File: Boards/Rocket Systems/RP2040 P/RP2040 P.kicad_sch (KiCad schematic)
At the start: 2 parts, among them J1 Conn_01x20_Pin, J3 Conn_01x18_Pin

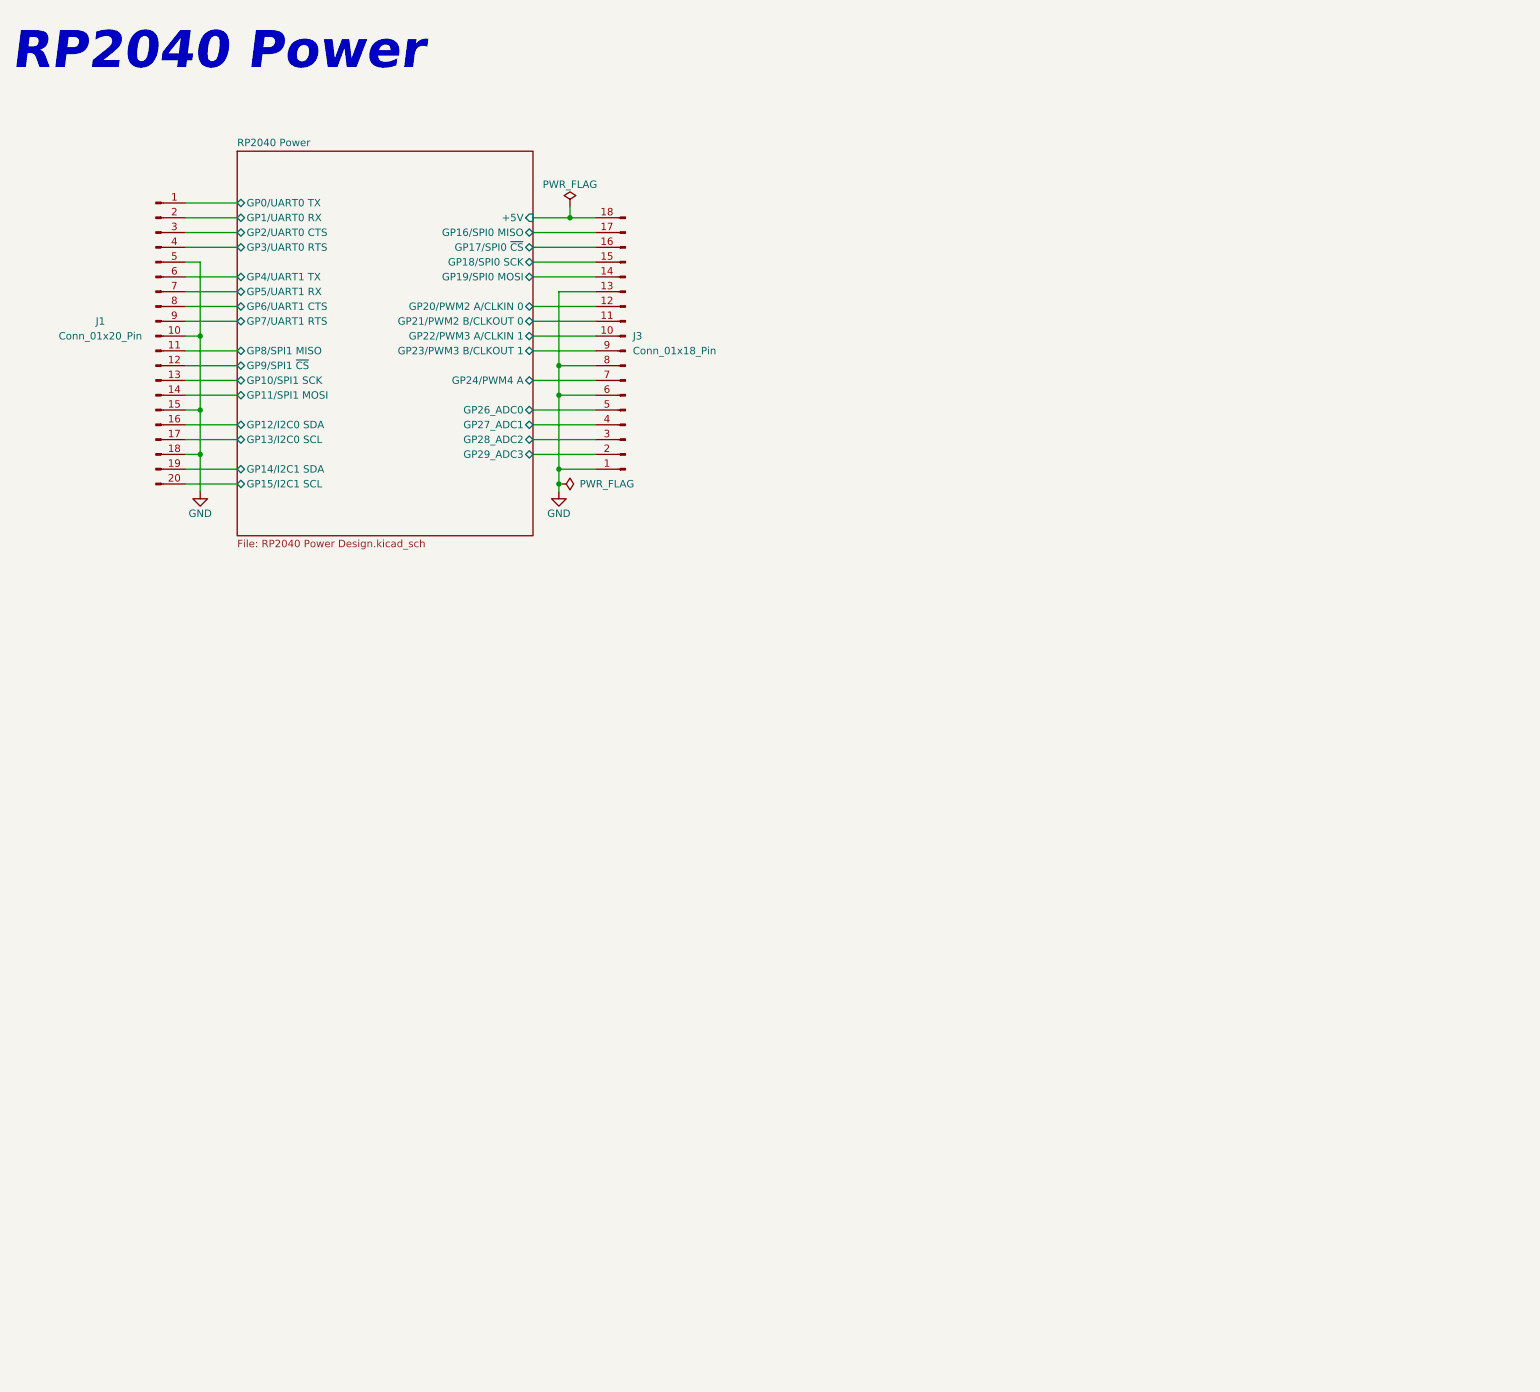
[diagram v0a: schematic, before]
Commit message: Alterações RP2040 P
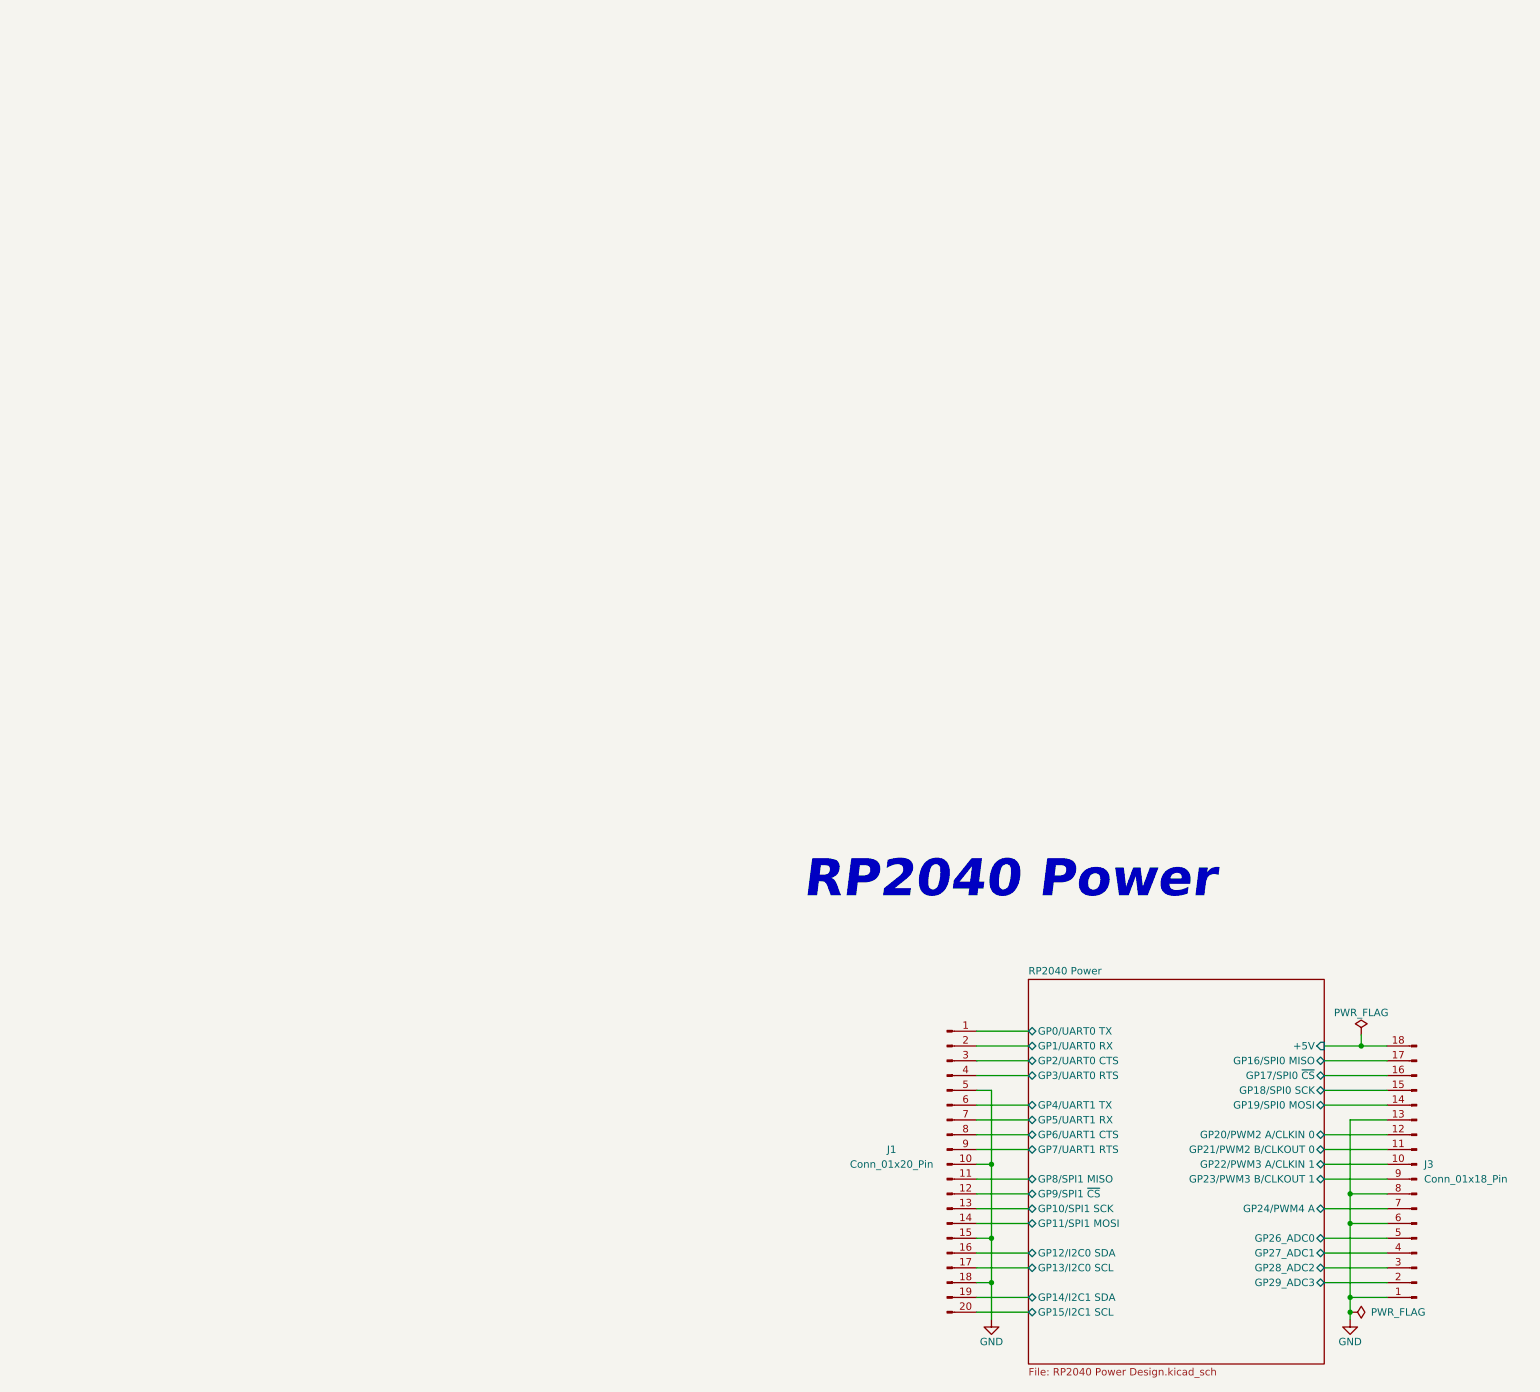
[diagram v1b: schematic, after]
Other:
- moved on the sheet: J1, J3
